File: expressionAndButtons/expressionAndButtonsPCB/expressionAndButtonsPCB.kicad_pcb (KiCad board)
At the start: 2 copper layers, 189.7 x 184.2 mm, 69 parts, among them J1 Alimentazione, J2 Conn_01x12, J3 OUTPUT Crescendo I, J4 OUTPUT EXPR I, J5 OUTPUT EXPR III, J6 INPUT C-I-III, J7 Conn_01x04, J8 OUTPUT Crescendo II, U2 ProMicro

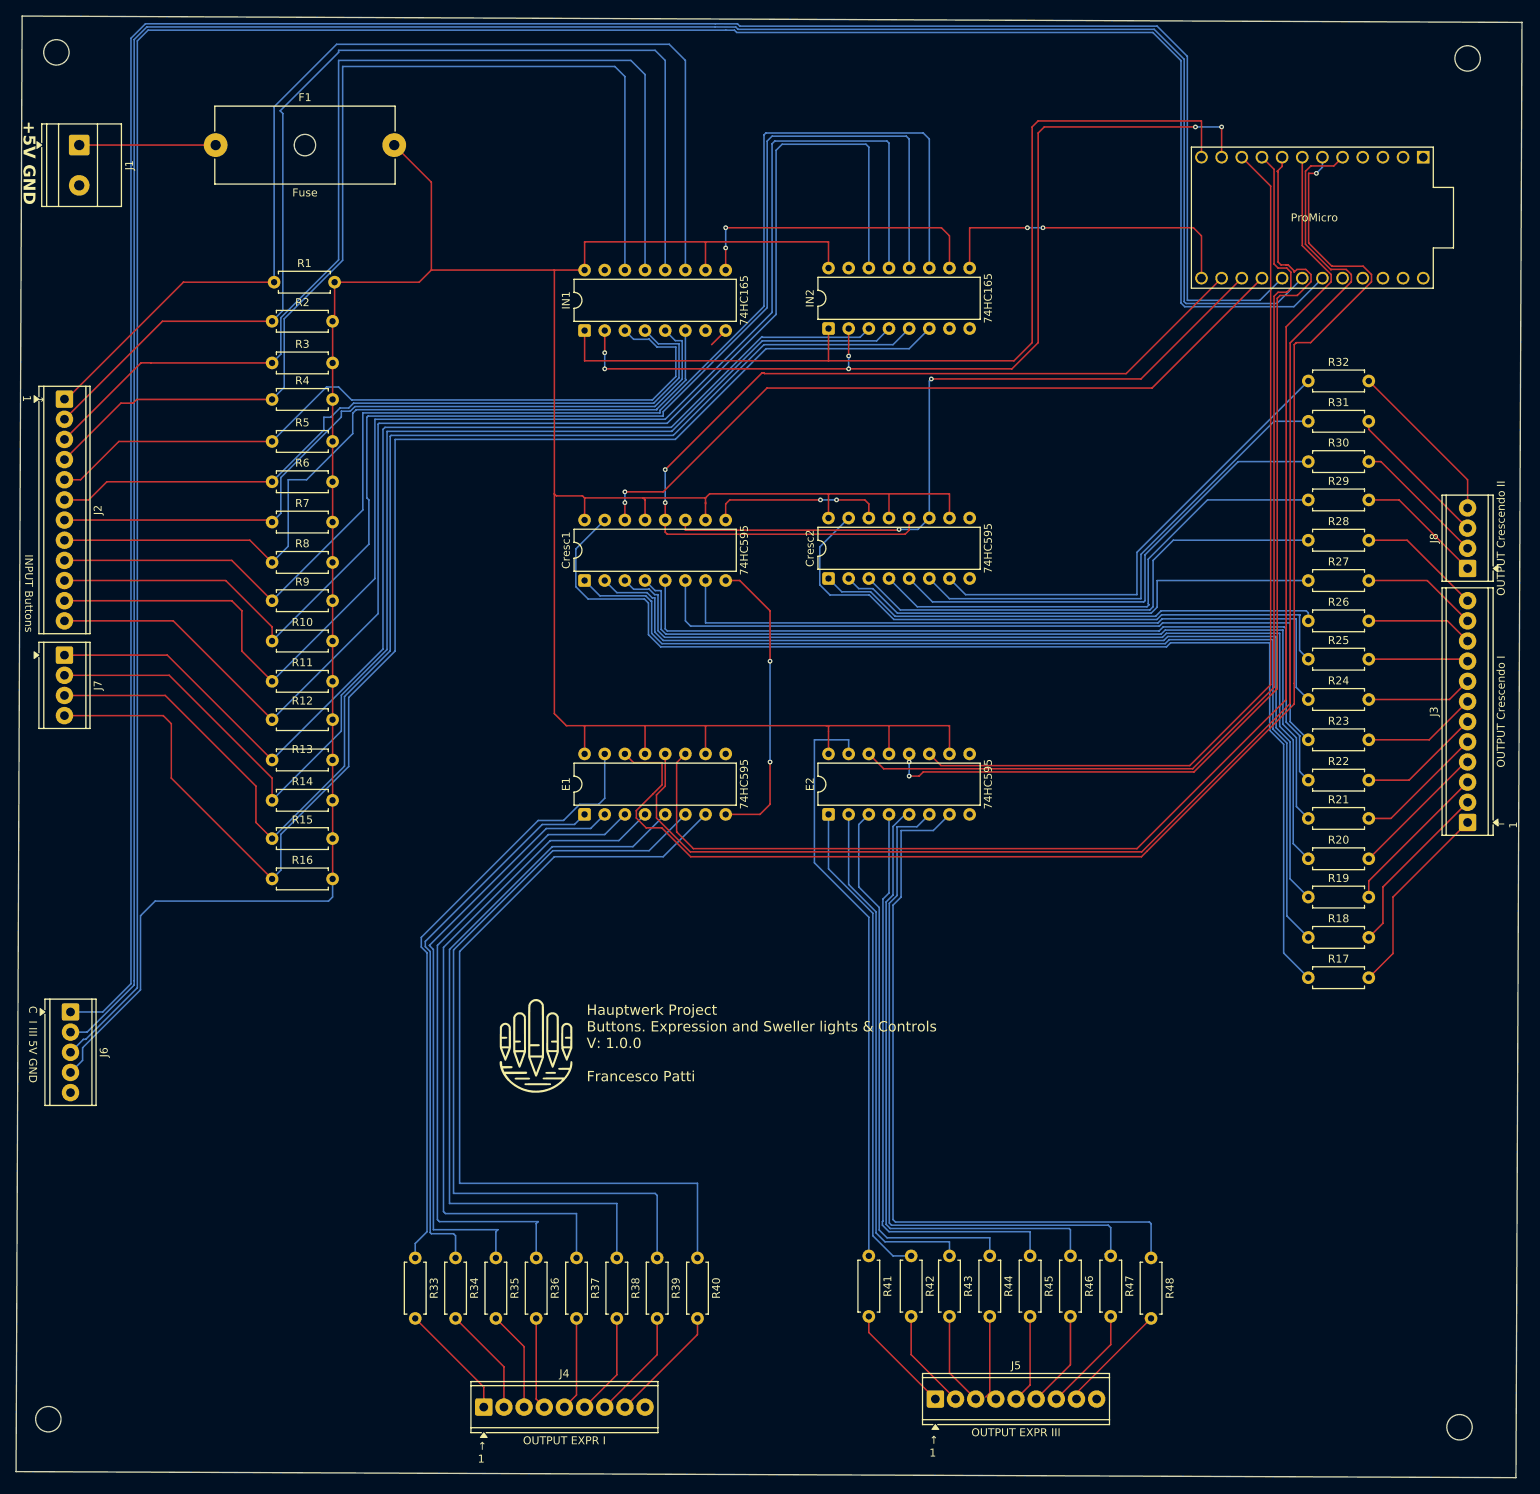
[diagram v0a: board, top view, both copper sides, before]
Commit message: update
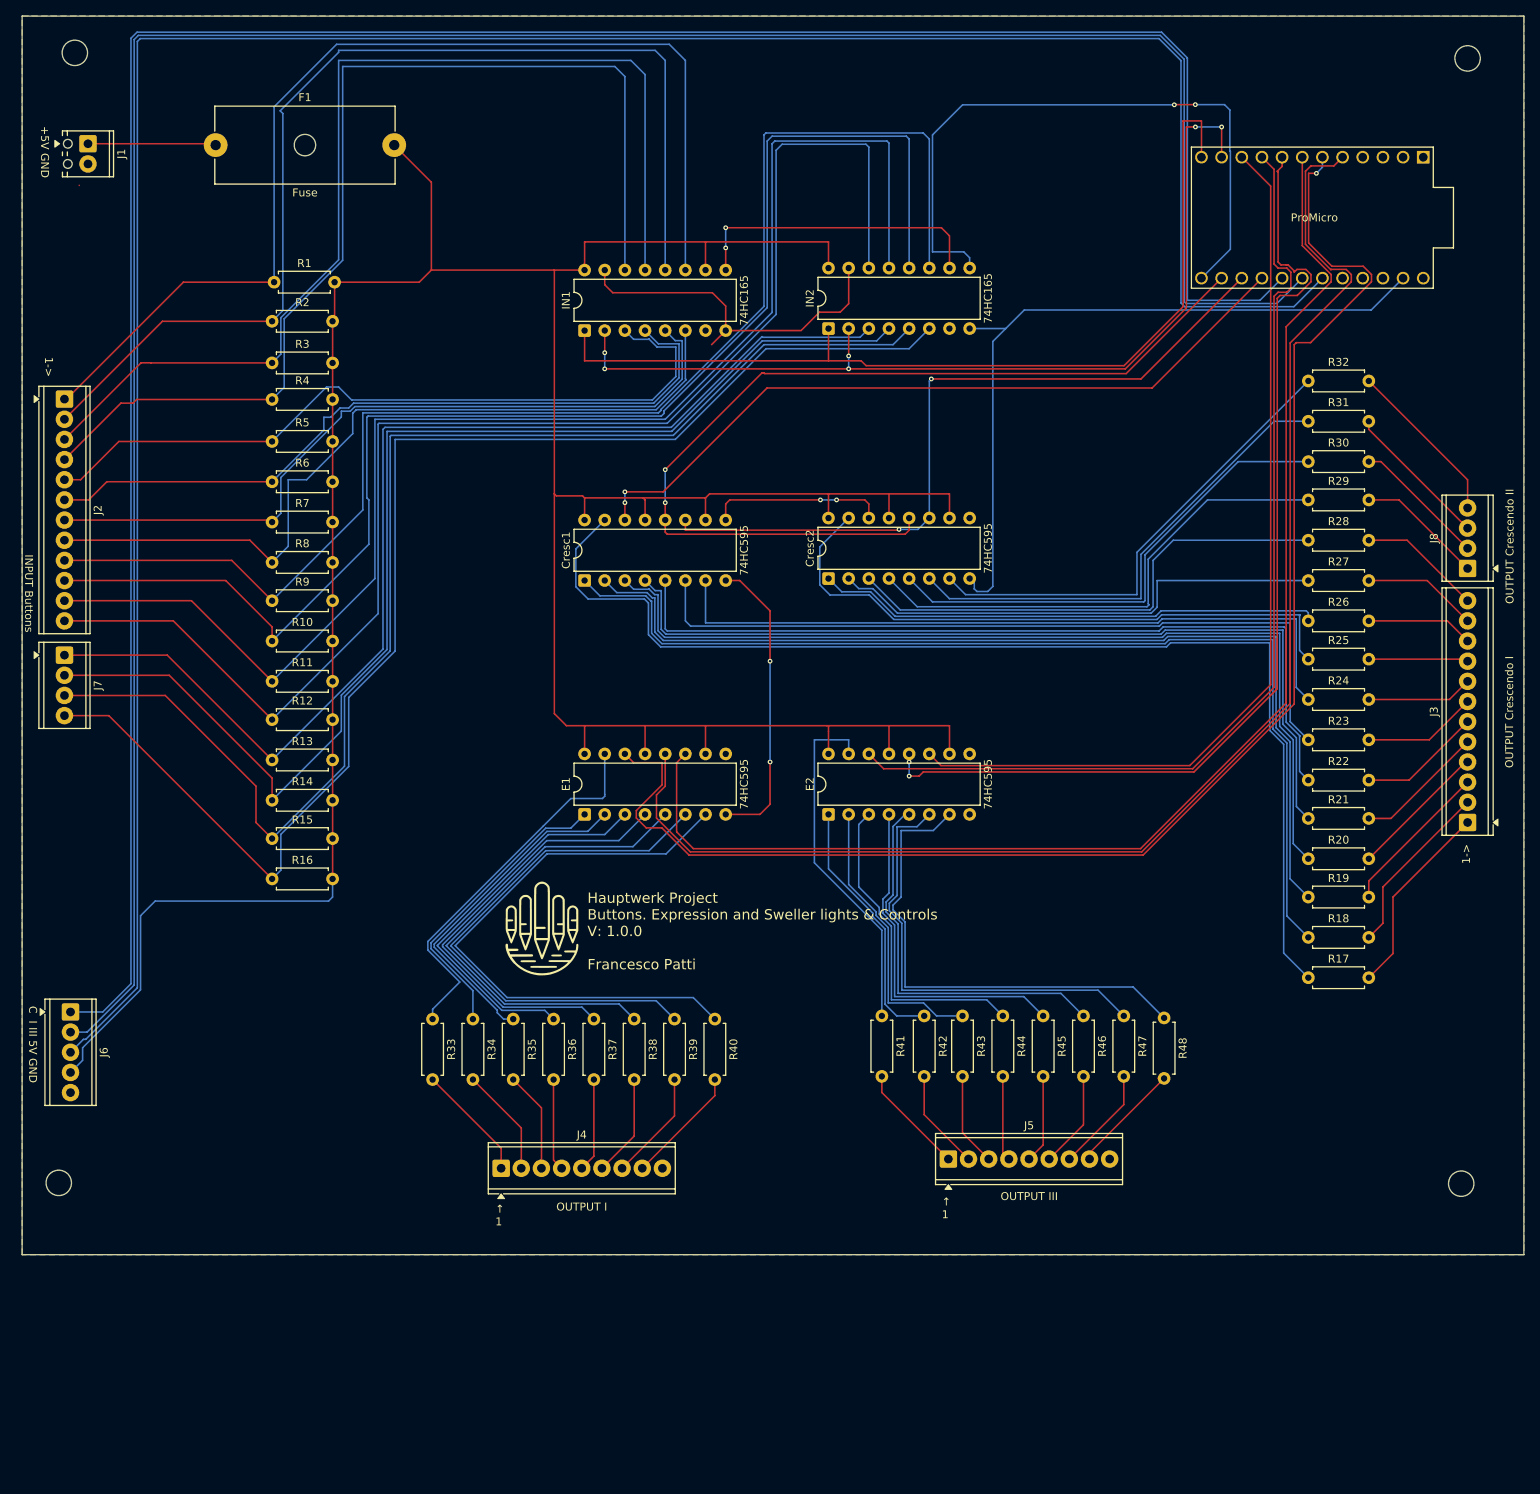
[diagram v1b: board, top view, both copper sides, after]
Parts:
- J1: footprint TerminalBlock_Phoenix:TerminalBlock_Phoenix_MKDS-1,5-2-5.08_1x02_P5.08mm_Horizontal -> TerminalBlock_Phoenix:TerminalBlock_Phoenix_MPT-0,5-2-2.54_1x02_P2.54mm_Horizontal
- J4: value OUTPUT EXPR I -> OUTPUT I
- J5: value OUTPUT EXPR III -> OUTPUT III
- moved REF** 30.7 mm to (213.6, 172.0)
- moved J5 30.3 mm to (149.0, 168.9)
- moved R41 30.3 mm to (140.6, 150.9)
- moved R42 30.3 mm to (145.9, 150.9)
- moved R43 30.3 mm to (150.7, 150.9)
- moved R44 30.3 mm to (155.8, 150.9)
- moved R45 30.3 mm to (160.9, 150.9)
- moved R46 30.3 mm to (166.0, 150.9)
- moved R47 30.3 mm to (171.1, 150.9)
- moved R48 30.3 mm to (176.1, 151.1)
- moved R33 30.2 mm to (84.0, 151.3)
- moved R34 30.2 mm to (89.1, 151.3)
- moved R35 30.2 mm to (94.1, 151.3)
- moved R36 30.2 mm to (99.2, 151.3)
- moved R37 30.2 mm to (104.3, 151.3)
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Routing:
- net GND: track 40.2 -> 177.5 mm
- net Net-(IN2-Q7): track 40.0 -> 83.1 mm
- net Net-(E1-QC): track 76.8 -> 42.5 mm
- net Net-(E1-QD): track 82.5 -> 49.0 mm
- net Net-(E1-QE): track 88.1 -> 55.4 mm
- net Net-(E1-QF): track 94.2 -> 62.0 mm
- net Net-(E1-QG): track 100.6 -> 68.5 mm
- net Net-(E1-QB): track 69.8 -> 37.8 mm
- net Net-(E1-QH): track 106.7 -> 74.9 mm
- net Net-(E2-QH): track 93.4 -> 62.0 mm
- net Net-(E2-QG): track 87.6 -> 56.5 mm
- net Net-(E2-QF): track 80.0 -> 49.2 mm
- net Net-(E2-QE): track 74.1 -> 43.6 mm
- net Net-(E2-QD): track 70.6 -> 40.5 mm
- net Net-(E2-QC): track 65.6 -> 35.9 mm
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- added copper zone on F.Cu, net GND
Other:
- board size 189.7 x 184.2 mm -> 189.2 x 156.1 mm
- board text added: "1->"
